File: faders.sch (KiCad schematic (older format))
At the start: 11 parts

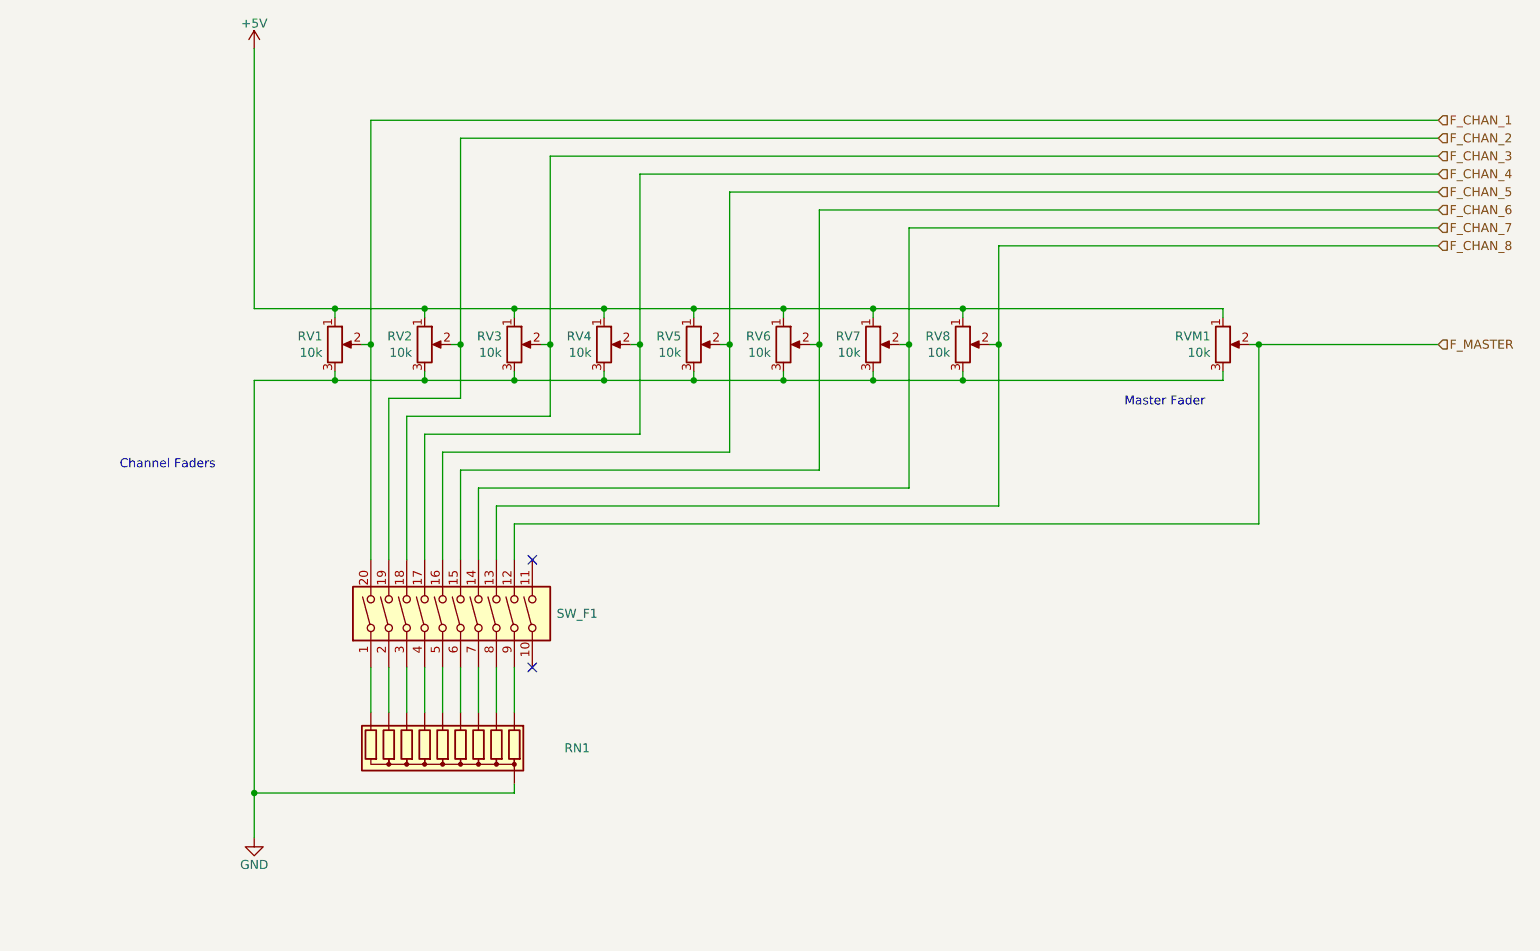
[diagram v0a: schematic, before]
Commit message: Sub boards completed
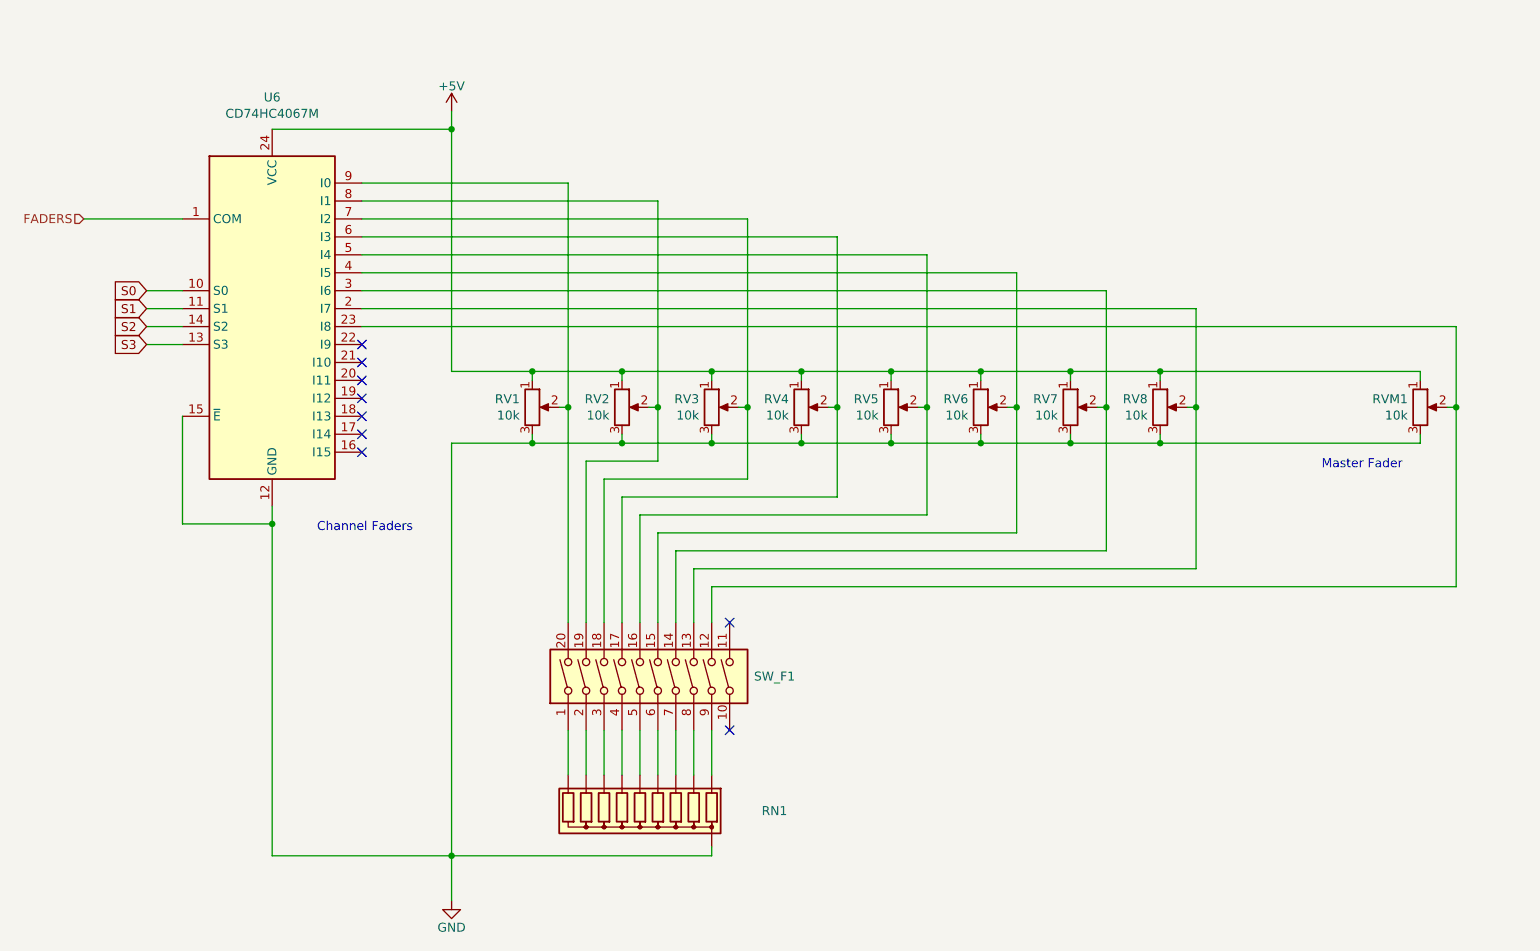
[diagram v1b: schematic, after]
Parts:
- added U6: CD74HC4067M, Package_SO:SOIC-24W_7.5x15.4mm_P1.27mm, symbol 74xx:CD74HC4067M
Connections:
- net +5V: now also U6.24 (VCC)
- net GND: now also U6.12 (GND), U6.15 (~E)
- net F_CHAN_1: no longer names the net of RV1.2, SW_F1.20
- net F_CHAN_1: now also U6.9 (I0)
- net F_CHAN_2: no longer names the net of RV2.2, SW_F1.19
- net F_CHAN_2: now also U6.8 (I1)
- net F_CHAN_3: no longer names the net of RV3.2, SW_F1.18
- net F_CHAN_3: now also U6.7 (I2)
- net F_CHAN_4: no longer names the net of RV4.2, SW_F1.17
- net F_CHAN_4: now also U6.6 (I3)
- net F_CHAN_5: no longer names the net of RV5.2, SW_F1.16
- net F_CHAN_5: now also U6.5 (I4)
- net F_CHAN_6: no longer names the net of RV6.2, SW_F1.15
- net F_CHAN_6: now also U6.4 (I5)
- net F_CHAN_7: no longer names the net of RV7.2, SW_F1.14
- net F_CHAN_7: now also U6.3 (I6)
- net F_CHAN_8: no longer names the net of RV8.2, SW_F1.13
- net F_CHAN_8: now also U6.2 (I7)
- net F_MASTER: no longer names the net of RVM1.2, SW_F1.12
- net F_MASTER: now also U6.23 (I8)
- new net FADERS: U6.1 (COM)
- new net S0: U6.10 (S0)
- new net S1: U6.11 (S1)
- new net S2: U6.14 (S2)
- new net S3: U6.13 (S3)
- no-connect marks 2 -> 9
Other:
- moved on the sheet: RN1, RV1, RV2, RV3, RV4, RV5, RV6, RV7, RV8, RVM1, SW_F1
